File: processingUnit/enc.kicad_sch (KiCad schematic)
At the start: 15 parts, among them J301 Conn_01x04, SW301 ENC RST, U301 STM32F401C_B-C_Ux, Y301 16Mhz

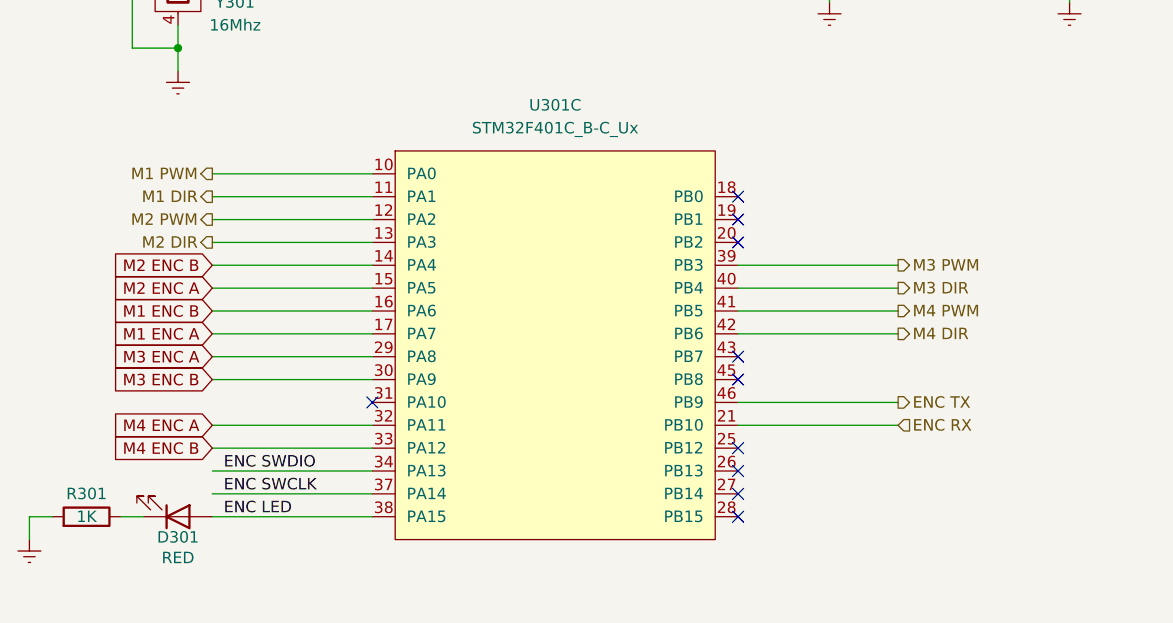
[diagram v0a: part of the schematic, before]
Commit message: drivers
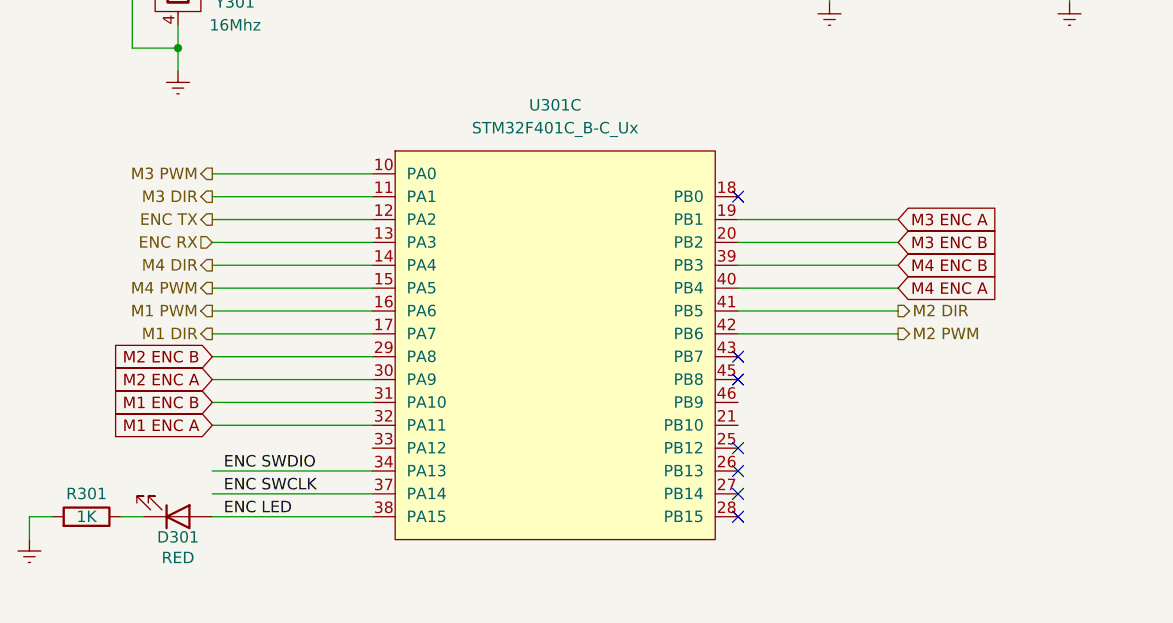
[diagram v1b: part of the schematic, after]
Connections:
- net ENC RX: now also U301.13 (PA3); no longer U301.21 (PB10)
- net ENC TX: now also U301.12 (PA2); no longer U301.46 (PB9)
- net M1 DIR: now also U301.17 (PA7); no longer U301.11 (PA1)
- net M1 ENC A: now also U301.32 (PA11); no longer U301.17 (PA7)
- net M1 ENC B: now also U301.31 (PA10); no longer U301.16 (PA6)
- net M1 PWM: now also U301.16 (PA6); no longer U301.10 (PA0)
- net M2 DIR: now also U301.41 (PB5); no longer U301.13 (PA3)
- net M2 ENC A: now also U301.30 (PA9); no longer U301.15 (PA5)
- net M2 ENC B: now also U301.29 (PA8); no longer U301.14 (PA4)
- net M2 PWM: now also U301.42 (PB6); no longer U301.12 (PA2)
- net M3 DIR: now also U301.11 (PA1); no longer U301.40 (PB4)
- net M3 ENC A: now also U301.19 (PB1); no longer U301.29 (PA8)
- net M3 ENC B: now also U301.20 (PB2); no longer U301.30 (PA9)
- net M3 PWM: now also U301.10 (PA0); no longer U301.39 (PB3)
- net M4 DIR: now also U301.14 (PA4); no longer U301.42 (PB6)
- net M4 ENC A: now also U301.40 (PB4); no longer U301.32 (PA11)
- net M4 ENC B: now also U301.39 (PB3); no longer U301.33 (PA12)
- net M4 PWM: now also U301.15 (PA5); no longer U301.41 (PB5)
- no-connect marks 13 -> 10

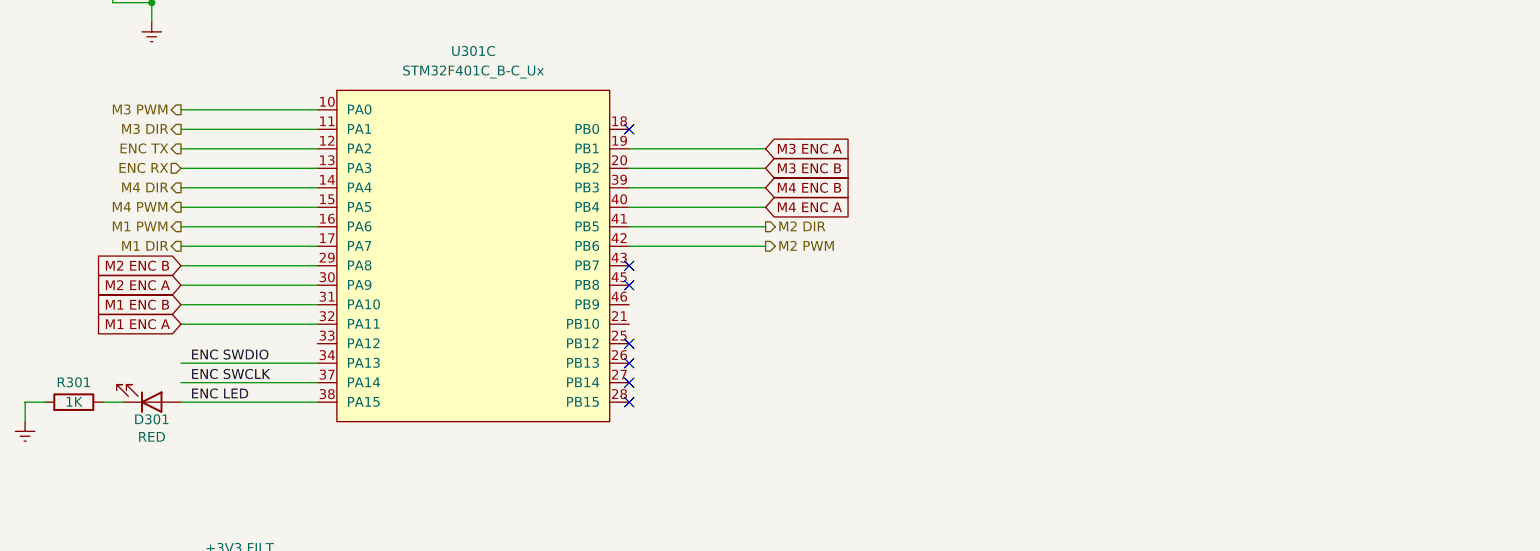
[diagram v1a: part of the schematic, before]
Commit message: l3 routing
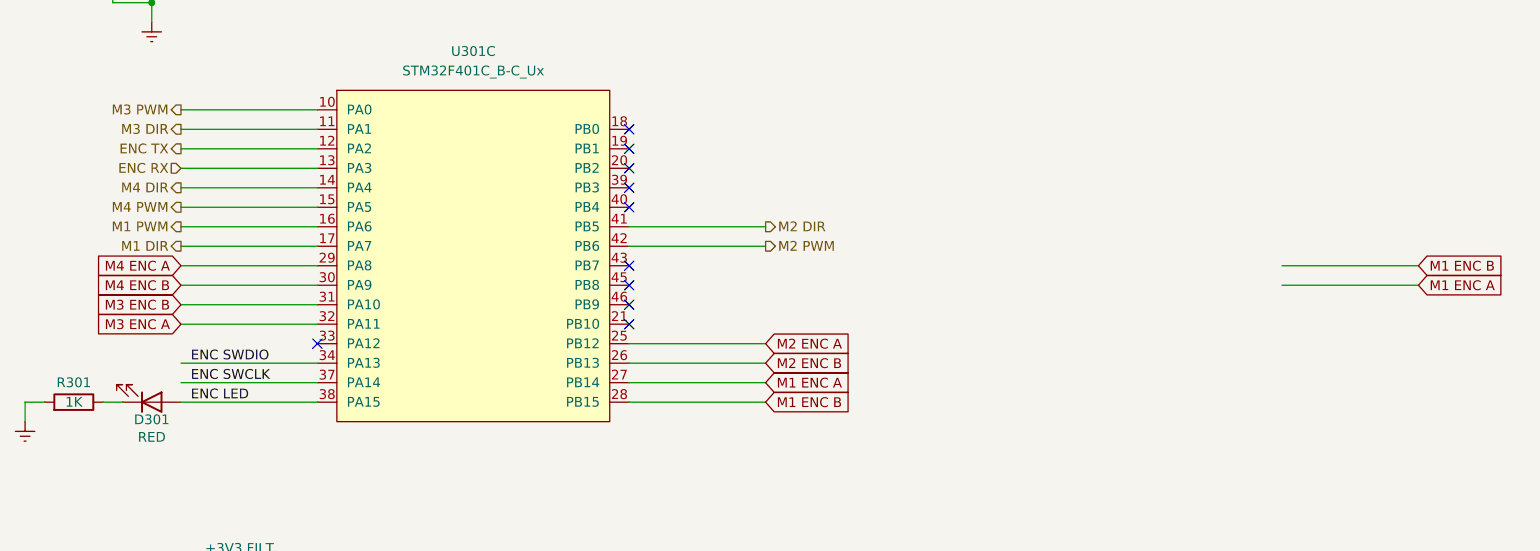
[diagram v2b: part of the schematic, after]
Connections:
- net M1 ENC A: now also U301.27 (PB14); no longer U301.32 (PA11)
- net M1 ENC B: now also U301.28 (PB15); no longer U301.31 (PA10)
- net M2 ENC A: now also U301.25 (PB12); no longer U301.30 (PA9)
- net M2 ENC B: now also U301.26 (PB13); no longer U301.29 (PA8)
- net M3 ENC A: now also U301.32 (PA11); no longer U301.19 (PB1)
- net M3 ENC B: now also U301.31 (PA10); no longer U301.20 (PB2)
- net M4 ENC A: now also U301.29 (PA8); no longer U301.40 (PB4)
- net M4 ENC B: now also U301.30 (PA9); no longer U301.39 (PB3)
- no-connect marks 10 -> 13

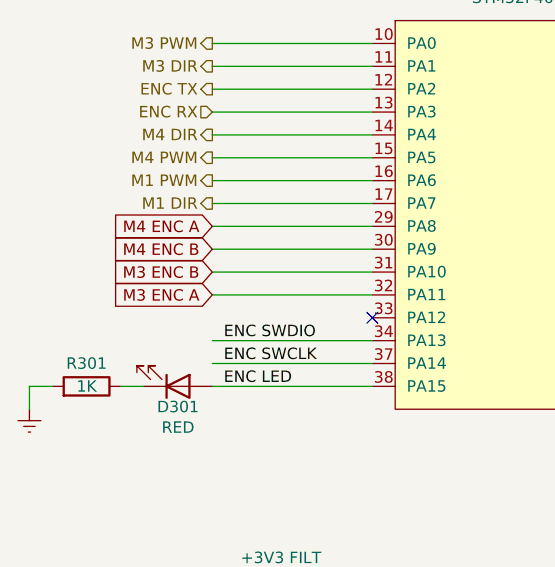
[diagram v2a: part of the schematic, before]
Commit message: logo
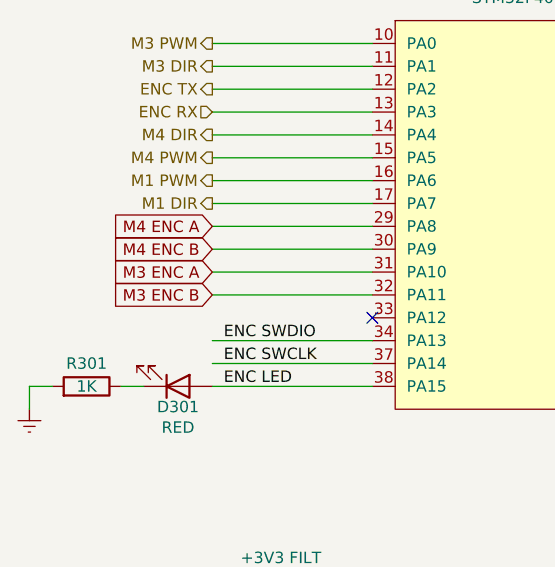
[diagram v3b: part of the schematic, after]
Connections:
- net M3 ENC A: now also U301.31 (PA10); no longer U301.32 (PA11)
- net M3 ENC B: now also U301.32 (PA11); no longer U301.31 (PA10)
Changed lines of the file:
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@@
 	(global_label "M3 ENC A"
 		(shape input)
+		(at 115.57 134.62 180)
+		(fields_autoplaced yes)
+		(effects
+			(font
+				(size 1.27 1.27)
+			)
+			(justify right)
+		)
+		(property "Intersheetrefs" "${INTERSHEET_REFS}"
+			(at 103.1506 134.62 0)
+			(effects
+				(font
+					(size 1.27 1.27)
+				)
+				(justify right)
+				(hide yes)
+			)
+		)
+	)
+	(global_label "M1 ENC A"
+		(shape input)
+		(at 191.77 144.78 0)
+		(fields_autoplaced yes)
+		(effects
+			(font
+				(size 1.27 1.27)
+			)
+			(justify left)
+		)
+		(property "Intersheetrefs" "${INTERSHEET_REFS}"
+			(at 204.1894 144.78 0)
+			(effects
+				(font
+					(size 1.27 1.27)
+				)
+				(justify left)
+				(hide yes)
+			)
+		)
+	)
+	(global_label "M4 ENC A"
+		(shape input)
+		(at 115.57 129.54 180)
+		(fields_autoplaced yes)
+		(effects
+			(font
+				(size 1.27 1.27)
+			)
+			(justify right)
+		)
+		(property "Intersheetrefs" "${INTERSHEET_REFS}"
+			(at 103.1506 129.54 0)
+			(effects
+				(font
+					(size 1.27 1.27)
+				)
+				(justify right)
+				(hide yes)
+			)
+		)
+	)
+	(global_label "M1 ENC B"
+		(shape input)
+		(at 191.77 147.32 0)
+		(fields_autoplaced yes)
+		(effects
+			(font
+				(size 1.27 1.27)
+			)
+			(justify left)
+		)
+		(property "Intersheetrefs" "${INTERSHEET_REFS}"
+			(at 204.3708 147.32 0)
+			(effects
+				(font
+					(size 1.27 1.27)
+				)
+				(justify left)
+				(hide yes)
+			)
+		)
+	)
+	(global_label "M1 ENC A"
+		(shape input)
+		(at 276.86 132.08 0)
+		(fields_autoplaced yes)
+		(effects
+			(font
+				(size 1.27 1.27)
+			)
+			(justify left)
+		)
+		(property "Intersheetrefs" "${INTERSHEET_REFS}"
+			(at 289.2794 132.08 0)
+			(effects
+				(font
+					(size 1.27 1.27)
+				)
+				(justify left)
+				(hide yes)
+			)
+		)
+	)
+	(global_label "M2 ENC B"
+		(shape input)
+		(at 191.77 142.24 0)
+		(fields_autoplaced yes)
+		(effects
+			(font
+				(size 1.27 1.27)
+			)
+			(justify left)
+		)
+		(property "Intersheetrefs" "${INTERSHEET_REFS}"
+			(at 204.3708 142.24 0)
+			(effects
+				(font
+					(size 1.27 1.27)
+				)
+				(justify left)
+				(hide yes)
+			)
+		)
+	)
+	(global_label "M1 ENC B"
+		(shape input)
+		(at 276.86 129.54 0)
+		(fields_autoplaced yes)
+		(effects
+			(font
+				(size 1.27 1.27)
+			)
+			(justify left)
+		)
+		(property "Intersheetrefs" "${INTERSHEET_REFS}"
+			(at 289.4608 129.54 0)
+			(effects
+				(font
+					(size 1.27 1.27)
+				)
+				(justify left)
+				(hide yes)
+			)
+		)
+	)
+	(global_label "M4 ENC B"
+		(shape input)
+		(at 115.57 132.08 180)
+		(fields_autoplaced yes)
+		(effects
+			(font
+				(size 1.27 1.27)
+			)
+			(justify right)
+		)
+		(property "Intersheetrefs" "${INTERSHEET_REFS}"
+			(at 102.9692 132.08 0)
+			(effects
+				(font
+					(size 1.27 1.27)
+				)
+				(justify right)
+				(hide yes)
+			)
+		)
+	)
+	(global_label "M2 ENC A"
+		(shape input)
+		(at 191.77 139.7 0)
+		(fields_autoplaced yes)
+		(effects
+			(font
+				(size 1.27 1.27)
+			)
+			(justify left)
+		)
+		(property "Intersheetrefs" "${INTERSHEET_REFS}"
+			(at 204.1894 139.7 0)
+			(effects
+				(font
+					(size 1.27 1.27)
+				)
+				(justify left)
+				(hide yes)
+			)
+		)
+	)
+	(global_label "M3 ENC B"
+		(shape input)
 		(at 115.57 137.16 180)
 		(fields_autoplaced yes)
@@
 		)
 		(property "Intersheetrefs" "${INTERSHEET_REFS}"
-			(at 103.1506 137.16 0)
-			(effects
-				(font
-					(size 1.27 1.27)
-				)
-				(justify right)
-				(hide yes)
-			)
-		)
-	)
-	(global_label "M1 ENC A"
-		(shape input)
-		(at 191.77 144.78 0)
-		(fields_autoplaced yes)
-		(effects
-			(font
-				(size 1.27 1.27)
-			)
-			(justify left)
-		)
-		(property "Intersheetrefs" "${INTERSHEET_REFS}"
-			(at 204.1894 144.78 0)
-			(effects
-				(font
-					(size 1.27 1.27)
-				)
-				(justify left)
-				(hide yes)
-			)
-		)
-	)
-	(global_label "M4 ENC A"
-		(shape input)
-		(at 115.57 129.54 180)
-		(fields_autoplaced yes)
-		(effects
-			(font
-				(size 1.27 1.27)
-			)
-			(justify right)
-		)
-		(property "Intersheetrefs" "${INTERSHEET_REFS}"
-			(at 103.1506 129.54 0)
-			(effects
-				(font
-					(size 1.27 1.27)
-				)
-				(justify right)
-				(hide yes)
-			)
-		)
-	)
-	(global_label "M1 ENC B"
-		(shape input)
-		(at 191.77 147.32 0)
-		(fields_autoplaced yes)
-		(effects
-			(font
-				(size 1.27 1.27)
-			)
-			(justify left)
-		)
-		(property "Intersheetrefs" "${INTERSHEET_REFS}"
-			(at 204.3708 147.32 0)
-			(effects
-				(font
-					(size 1.27 1.27)
-				)
-				(justify left)
-				(hide yes)
-			)
-		)
-	)
-	(global_label "M1 ENC A"
-		(shape input)
-		(at 276.86 132.08 0)
-		(fields_autoplaced yes)
-		(effects
-			(font
-				(size 1.27 1.27)
-			)
-			(justify left)
-		)
-		(property "Intersheetrefs" "${INTERSHEET_REFS}"
-			(at 289.2794 132.08 0)
-			(effects
-				(font
-					(size 1.27 1.27)
-				)
-				(justify left)
-				(hide yes)
-			)
-		)
-	)
-	(global_label "M2 ENC B"
-		(shape input)
-		(at 191.77 142.24 0)
-		(fields_autoplaced yes)
-		(effects
-			(font
-				(size 1.27 1.27)
-			)
-			(justify left)
-		)
-		(property "Intersheetrefs" "${INTERSHEET_REFS}"
-			(at 204.3708 142.24 0)
-			(effects
-				(font
-					(size 1.27 1.27)
-				)
-				(justify left)
-				(hide yes)
-			)
-		)
-	)
-	(global_label "M1 ENC B"
-		(shape input)
-		(at 276.86 129.54 0)
-		(fields_autoplaced yes)
-		(effects
-			(font
-				(size 1.27 1.27)
-			)
-			(justify left)
-		)
-		(property "Intersheetrefs" "${INTERSHEET_REFS}"
-			(at 289.4608 129.54 0)
-			(effects
-				(font
-					(size 1.27 1.27)
-				)
-				(justify left)
-				(hide yes)
-			)
-		)
-	)
-	(global_label "M4 ENC B"
-		(shape input)
-		(at 115.57 132.08 180)
-		(fields_autoplaced yes)
-		(effects
-			(font
-				(size 1.27 1.27)
-			)
-			(justify right)
-		)
-		(property "Intersheetrefs" "${INTERSHEET_REFS}"
-			(at 102.9692 132.08 0)
-			(effects
-				(font
-					(size 1.27 1.27)
-				)
-				(justify right)
-				(hide yes)
-			)
-		)
-	)
-	(global_label "M2 ENC A"
-		(shape input)
-		(at 191.77 139.7 0)
-		(fields_autoplaced yes)
-		(effects
-			(font
-				(size 1.27 1.27)
-			)
-			(justify left)
-		)
-		(property "Intersheetrefs" "${INTERSHEET_REFS}"
-			(at 204.1894 139.7 0)
-			(effects
-				(font
-					(size 1.27 1.27)
-				)
-				(justify left)
-				(hide yes)
-			)
-		)
-	)
-	(global_label "M3 ENC B"
-		(shape input)
-		(at 115.57 134.62 180)
-		(fields_autoplaced yes)
-		(effects
-			(font
-				(size 1.27 1.27)
-			)
-			(justify right)
-		)
-		(property "Intersheetrefs" "${INTERSHEET_REFS}"
-			(at 102.9692 134.62 0)
-			(effects
-				(font
+			(at 102.9692 137.16 0)
+			(effects
+				(font

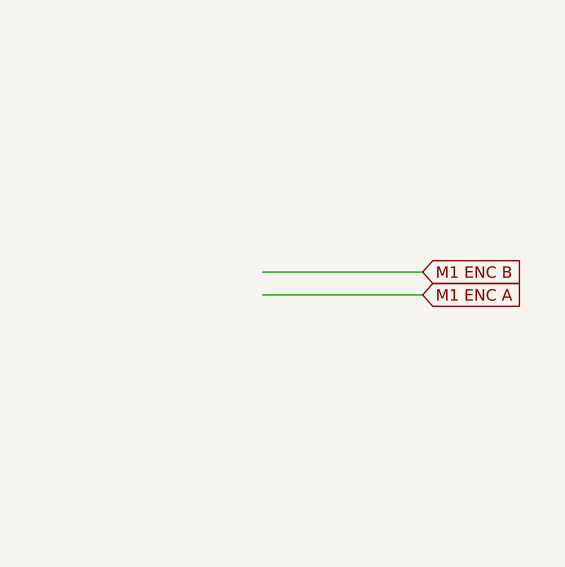
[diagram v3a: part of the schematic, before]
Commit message: step
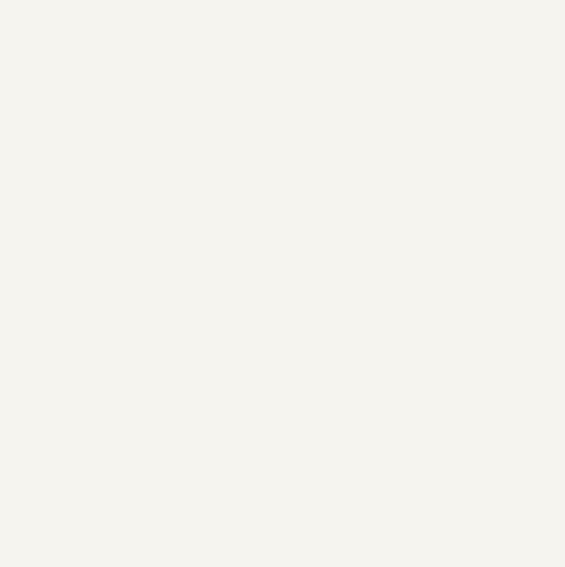
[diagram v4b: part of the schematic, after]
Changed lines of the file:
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@@
-	(wire
-		(pts
-			(xy 276.86 132.08) (xy 259.08 132.08)
-		)
-		(stroke
-			(width 0)
-			(type default)
-		)
-	)
 	(wire
 		(pts
@@
 		(pts
 			(xy 106.68 95.25) (xy 111.76 95.25)
-		)
-		(stroke
-			(width 0)
-			(type default)
-		)
-	)
-	(wire
-		(pts
-			(xy 276.86 129.54) (xy 259.08 129.54)
 		)
 		(stroke
@@
 		)
 	)
-	(global_label "M1 ENC A"
-		(shape input)
-		(at 276.86 132.08 0)
-		(fields_autoplaced yes)
-		(effects
-			(font
-				(size 1.27 1.27)
-			)
-			(justify left)
-		)
-		(property "Intersheetrefs" "${INTERSHEET_REFS}"
-			(at 289.2794 132.08 0)
-			(effects
-				(font
-					(size 1.27 1.27)
-				)
-				(justify left)
-				(hide yes)
-			)
-		)
-	)
 	(global_label "M2 ENC B"
 		(shape input)
@@
 			(effects
 				(font
-					(size 1.27 1.27)
-				)
-				(justify left)
-				(hide yes)
-			)
-		)
-	)
-	(global_label "M1 ENC B"
-		(shape input)
-		(at 276.86 129.54 0)
-		(fields_autoplaced yes)
-		(effects
-			(font
-				(size 1.27 1.27)
-			)
-			(justify left)
-		)
-		(property "Intersheetrefs" "${INTERSHEET_REFS}"
-			(at 289.4608 129.54 0)
-			(effects
-				(font

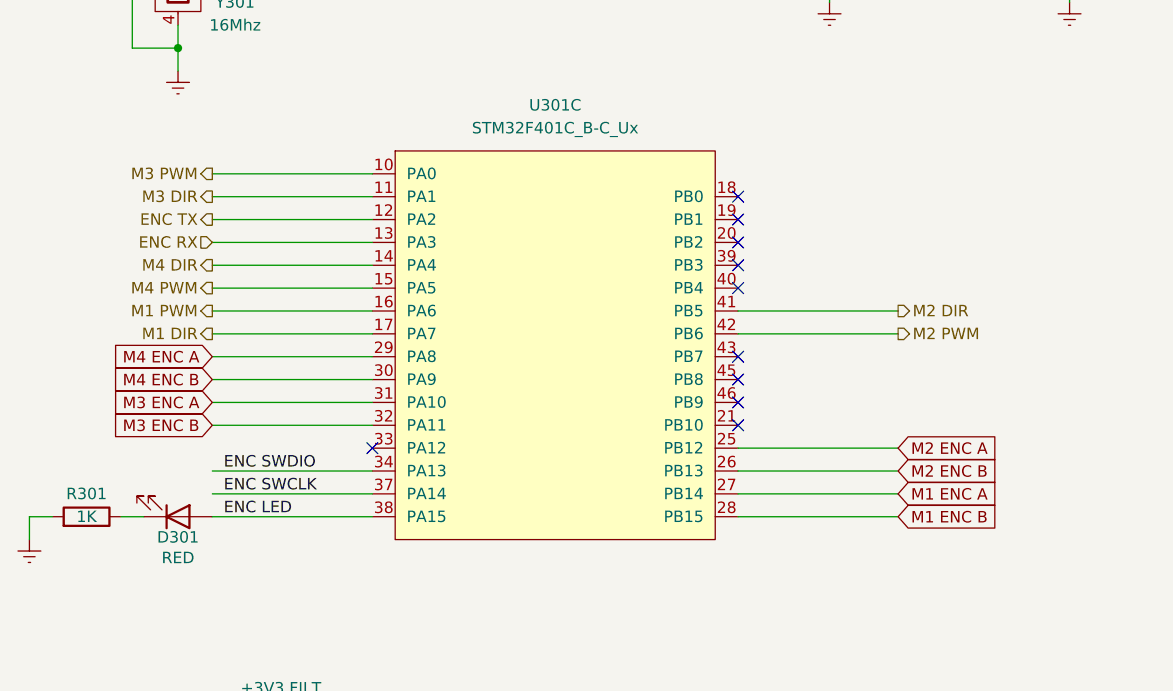
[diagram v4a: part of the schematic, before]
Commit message: nightmare fuel
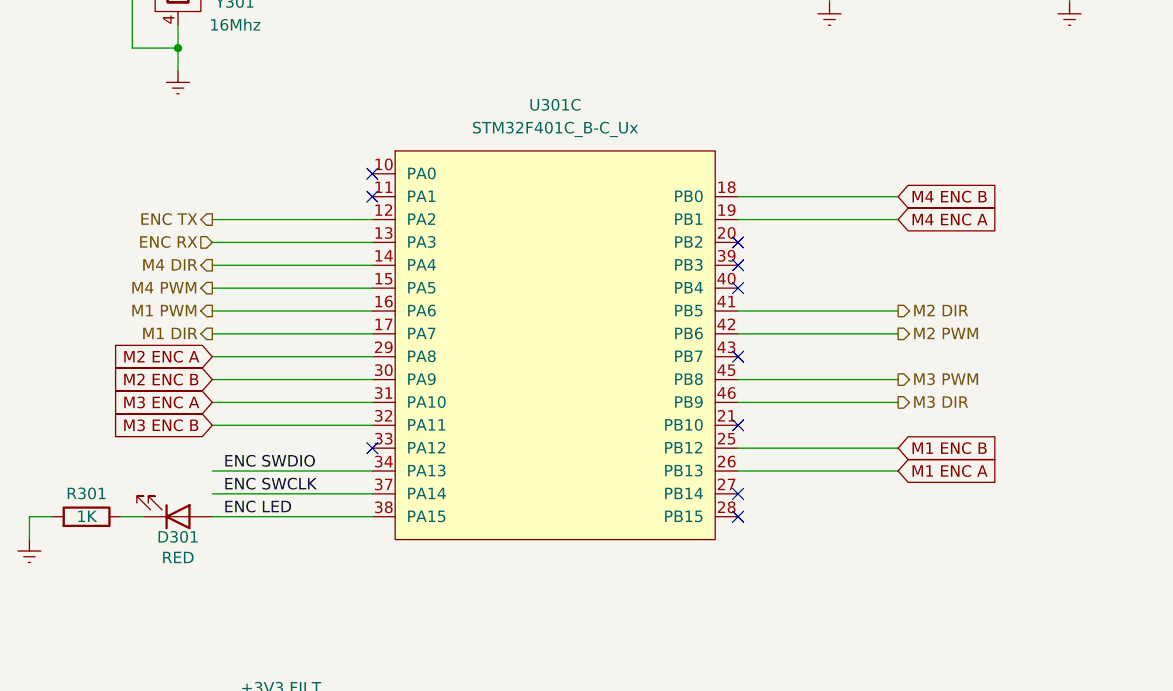
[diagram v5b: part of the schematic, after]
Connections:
- net M1 ENC A: now also U301.26 (PB13); no longer U301.27 (PB14)
- net M1 ENC B: now also U301.25 (PB12); no longer U301.28 (PB15)
- net M2 ENC A: now also U301.29 (PA8); no longer U301.25 (PB12)
- net M2 ENC B: now also U301.30 (PA9); no longer U301.26 (PB13)
- net M3 DIR: now also U301.46 (PB9); no longer U301.11 (PA1)
- net M3 PWM: now also U301.45 (PB8); no longer U301.10 (PA0)
- net M4 ENC A: now also U301.19 (PB1); no longer U301.29 (PA8)
- net M4 ENC B: now also U301.18 (PB0); no longer U301.30 (PA9)
